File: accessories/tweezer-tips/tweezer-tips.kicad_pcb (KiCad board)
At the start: 2 copper layers, 130 x 10 mm, 9 parts, among them J1 TIP, J2 TO_AMP, J3 GND

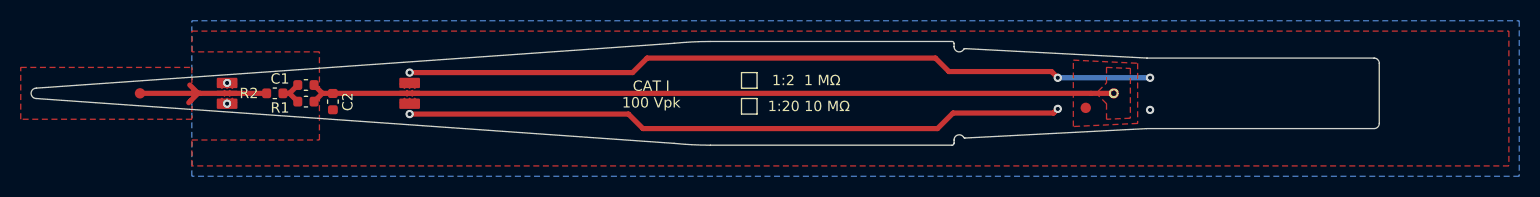
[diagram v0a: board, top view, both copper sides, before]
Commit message: Revision 4
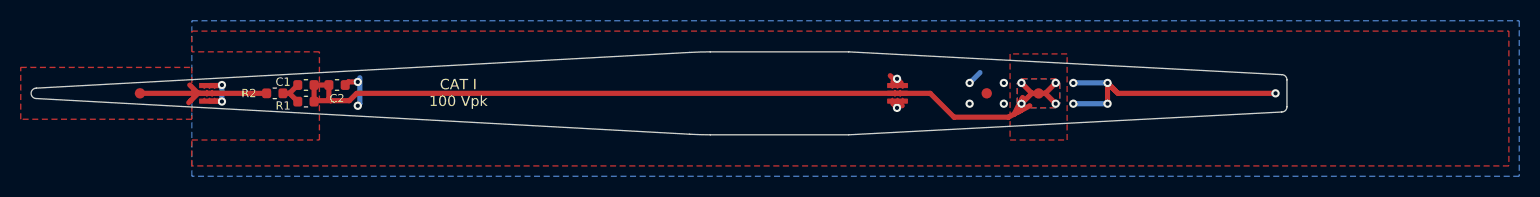
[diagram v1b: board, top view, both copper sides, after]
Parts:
- J2: footprint TestPoint:TestPoint_THTPad_D1.0mm_Drill0.5mm -> oscilloscope-probes:SIMPLE_PAD
- moved E2 47.1 mm to (208.1, 100.0)
- moved J3 9.65 mm to (216.7, 100.0)
- moved J2 7.25 mm to (221.7, 100.0)
- moved E1 1.70 mm to (141.7, 100.0)
- moved C2 1.65 mm to (154.0, 99.2), turned to 0 degrees
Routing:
- net GND: track 136.7 -> 40.2 mm, vias 8 -> 15
- net /AMP: track 78.6 -> 86.3 mm, vias 0 -> 4
- added copper zone on B.Cu, net /AMP
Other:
- board size 130 x 10 mm -> 121.1 x 8 mm
- board text added: "Enclosure front edge"
- board text removed: "1:2 1 MΩ"
- board text removed: "1:20 10 MΩ"
- board text removed: "Main pcb front edge"
